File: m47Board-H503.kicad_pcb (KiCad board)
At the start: 4 copper layers, 40 x 34 mm, 44 parts, among them J1 USB_C_Receptacle_USB2.0_16P, J3 Conn_01x15_Pin, J4 Conn_01x10_Pin, J5 Conn_01x15_Pin, SW1 SW_Push, SW2 SW_Push, SW3 SW_Push, U1 AP2114HA-3.3TRG1, U2 STM32H503CBTx, U3 USBLC6-2SC6, Y1 CX3225FB16000F0FZZH1 16MHz, Y2 ABS07-32.768KHZ-T

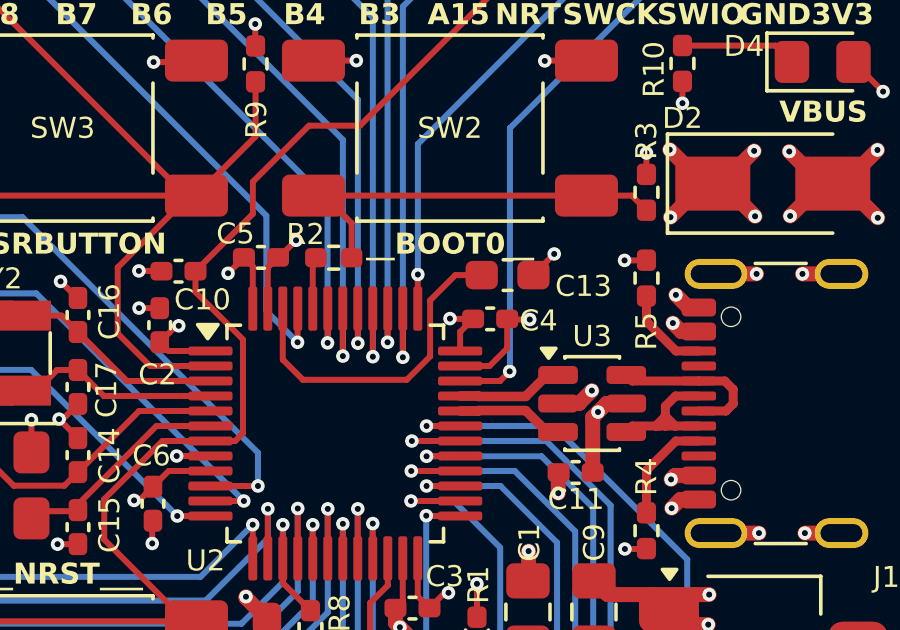
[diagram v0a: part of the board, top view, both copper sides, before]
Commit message: Move cap
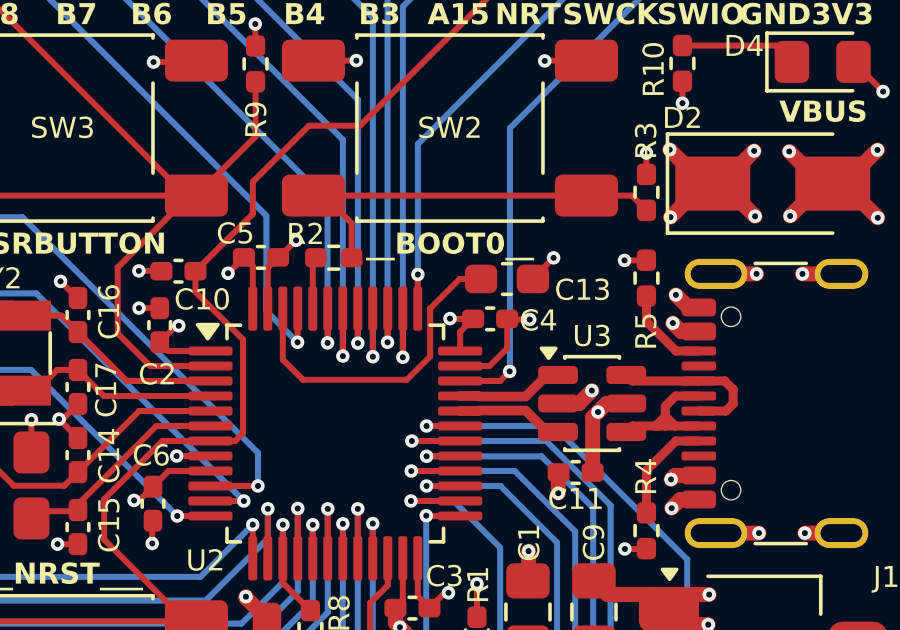
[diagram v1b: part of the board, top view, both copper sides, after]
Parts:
- moved C13 0.13 mm to (146.2, 98.7)
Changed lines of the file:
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@@
 	(footprint "Capacitor_SMD:C_0603_1608Metric_Pad1.08x0.95mm_HandSolder"
 		(layer "F.Cu")
-		(at 146.27 98.58)
+		(at 146.25 98.71)
 		(descr "Capacitor SMD 0603 (1608 Metric), square (rectangular) end terminal, IPC-7351 nominal with elongated pad for handsoldering. (Body size source: IPC-SM-782 page 76, https://www.pcb-3d.com/wordpress/wp-content/uploads/ipc-sm-782a_amendment_1_and_2.pdf)")
 		(tags "capacitor handsolder")
@@
 	)
 	(segment
-		(start 147.825 97.875)
-		(end 147.16 98.54)
+		(start 147.805 98.005)
+		(end 147.14 98.67)
 		(width 0.2)
 		(layer "F.Cu")
@@
 	)
 	(via
-		(at 147.825 97.875)
+		(at 147.805 98.005)
 		(size 0.45)
 		(drill 0.2)
@@
 	)
 	(segment
-		(start 139.45 102.07)
+		(start 138.7775 99.6975)
 		(end 138.7775 101.3975)
 		(width 0.2)
@@
 	)
 	(segment
-		(start 144.53 98.58)
-		(end 143.69 99.42)
+		(start 138.7775 101.3975)
+		(end 139.45 102.07)
 		(width 0.2)
 		(layer "F.Cu")
@@
 	)
 	(segment
-		(start 142.91 102.07)
-		(end 139.45 102.07)
+		(start 143.69 101.29)
+		(end 143.69 99.69)
 		(width 0.2)
 		(layer "F.Cu")
@@
 	)
 	(segment
-		(start 145.4075 98.58)
-		(end 144.53 98.58)
+		(start 139.45 102.07)
+		(end 142.91 102.07)
 		(width 0.2)
 		(layer "F.Cu")
@@
 	)
 	(segment
-		(start 138.7775 101.3975)
-		(end 138.7775 99.6975)
+		(start 142.91 102.07)
+		(end 143.69 101.29)
 		(width 0.2)
 		(layer "F.Cu")
@@
 	)
 	(segment
-		(start 143.69 99.42)
-		(end 143.69 101.29)
+		(start 143.69 99.69)
+		(end 144.67 98.71)
 		(width 0.2)
 		(layer "F.Cu")
@@
 	)
 	(segment
-		(start 143.69 101.29)
-		(end 142.91 102.07)
+		(start 144.67 98.71)
+		(end 145.3875 98.71)
 		(width 0.2)
 		(layer "F.Cu")
